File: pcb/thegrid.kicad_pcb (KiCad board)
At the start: 2 copper layers, 49.8 x 99.8 mm, 54 parts, among them P1 POWER, P10 CONN_2, P2 SHIFT_IN, P3 SHIFT_OUT, P4 CONN_2, P5 CONN_2, P6 CONN_2, P7 CONN_2, P8 CONN_2, P9 CONN_2, Q1 FQP7P06, Q2 FQP7P06, Q3 FQP7P06, Q4 FQP7P06, Q5 FQP7P06, Q6 FQP7P06, Q7 FQP7P06, U1 UA7805CKCS, U2 TPIC6C595

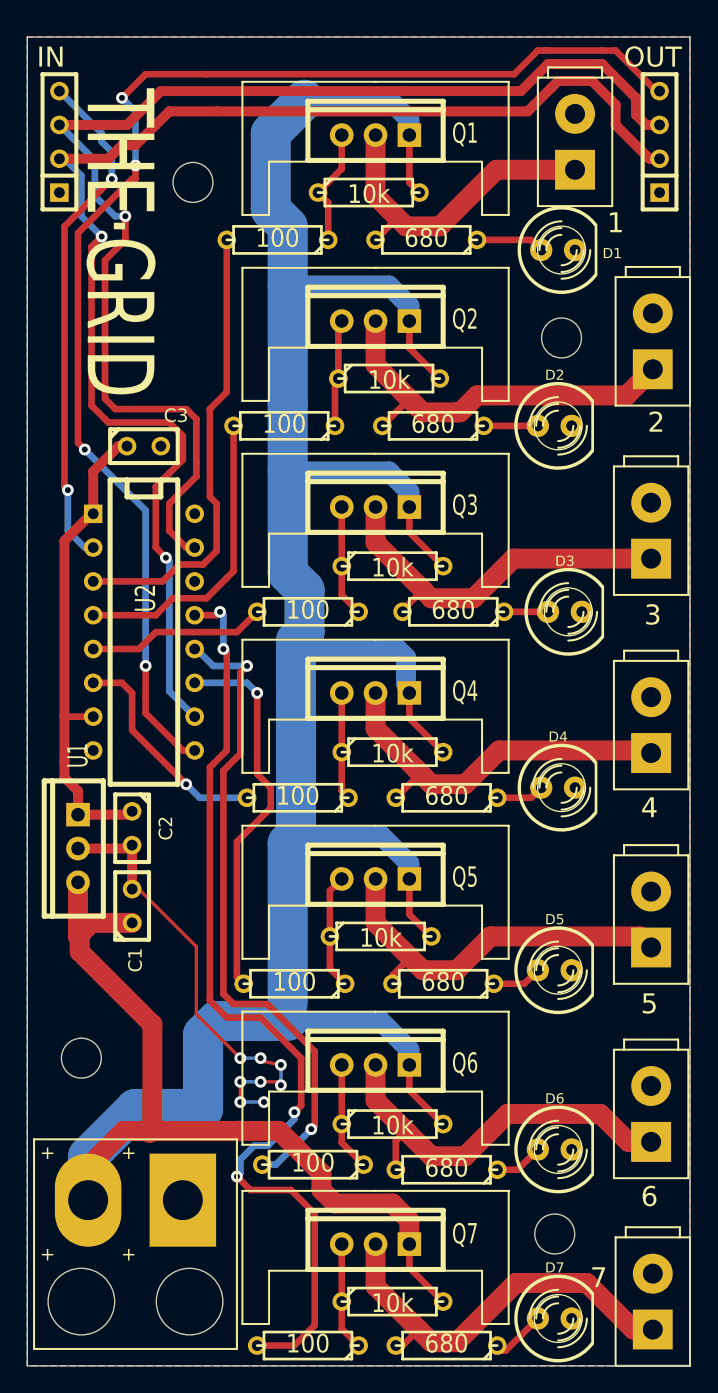
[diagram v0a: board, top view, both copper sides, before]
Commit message: Bumped via size
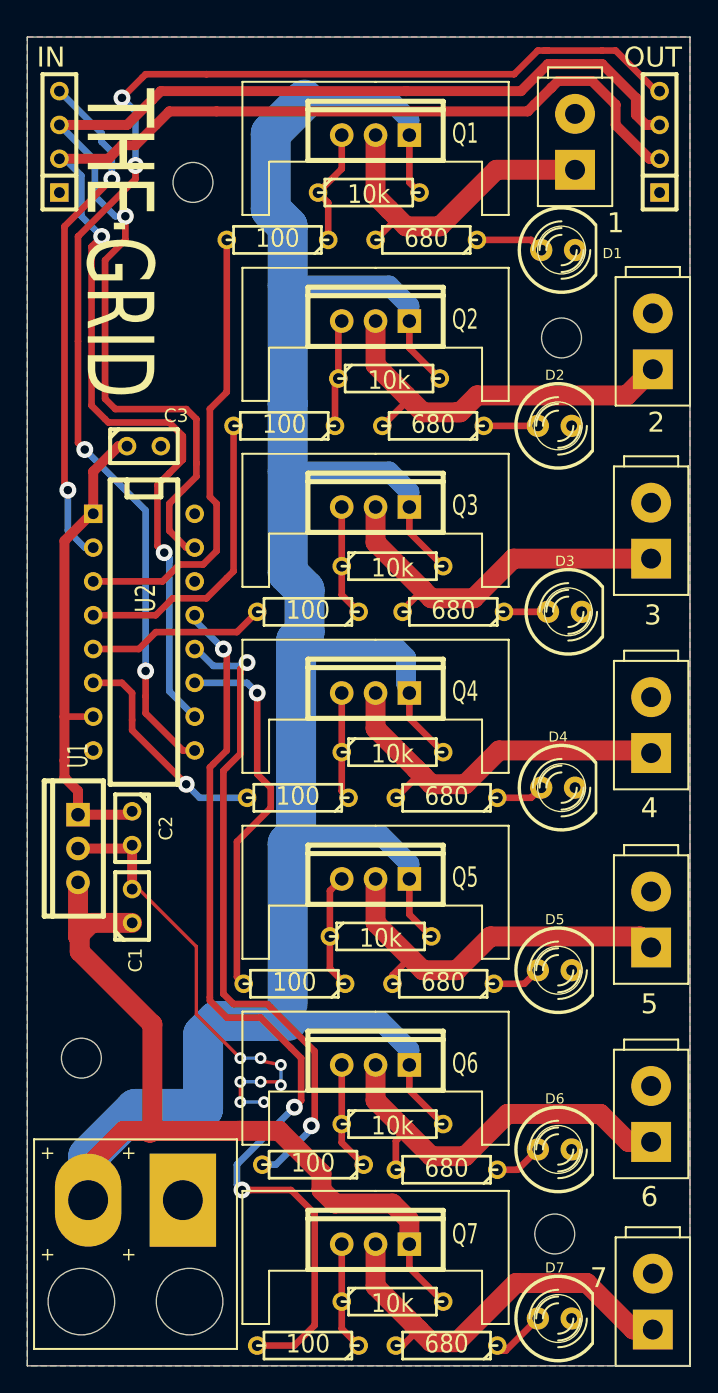
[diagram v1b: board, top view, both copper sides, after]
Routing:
- net Net-(R12-Pad2): track 72.4 -> 70.7 mm, vias 4 -> 3
